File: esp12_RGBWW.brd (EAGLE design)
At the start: 53 x 47 mm, 36 parts, among them Q1 AOD2910SMD, Q2 AOD2910SMD, Q3 AOD2910SMD, Q4 AOD2910SMD, Q5 AOD2910SMD, U1 TPS5410DR

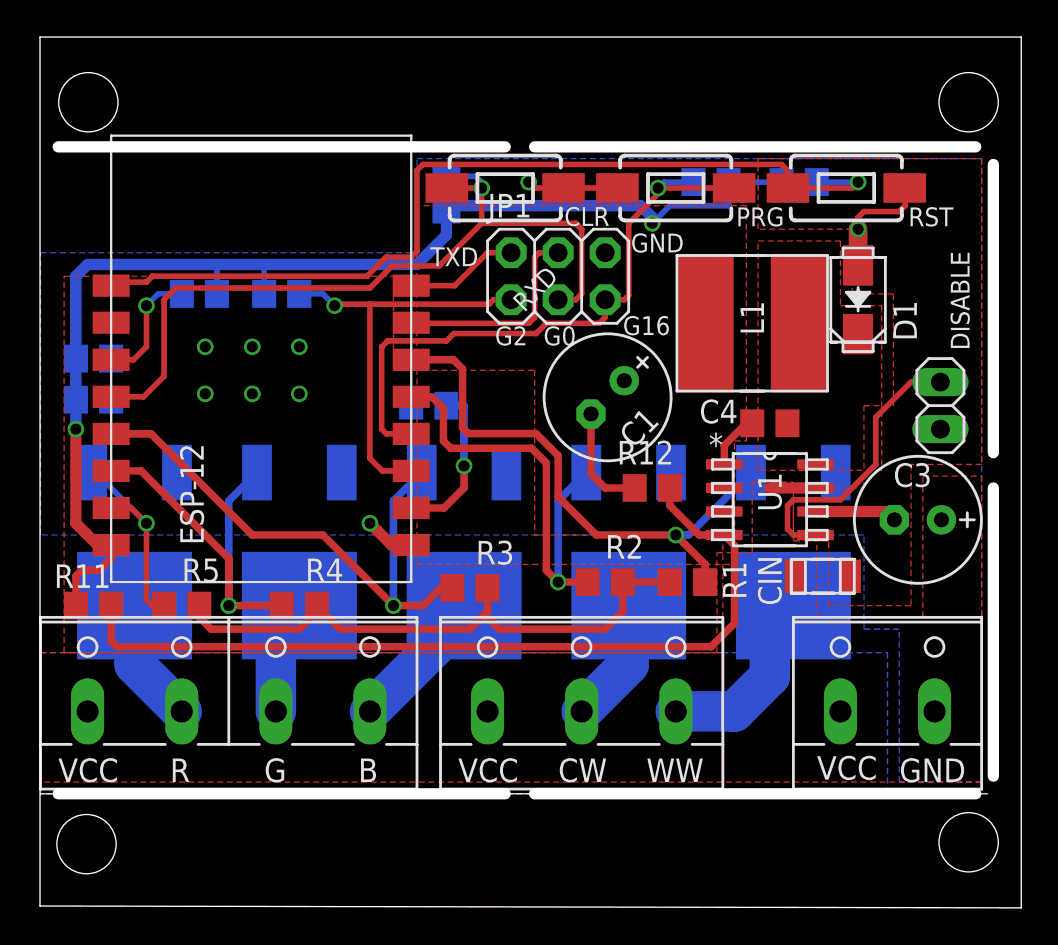
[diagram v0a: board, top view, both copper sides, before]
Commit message: small changes
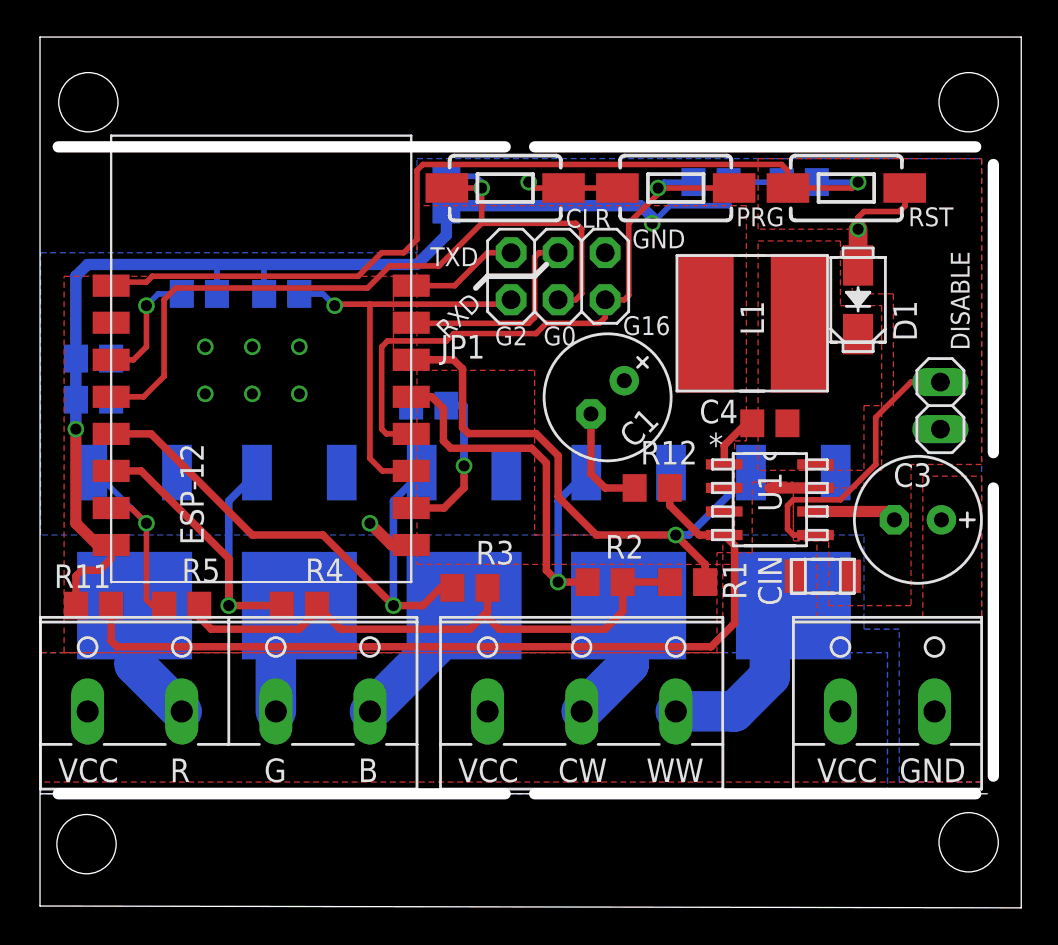
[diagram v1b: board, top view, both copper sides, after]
